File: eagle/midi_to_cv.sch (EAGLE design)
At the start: 36 parts, among them IC1 TL074P, IC4 TL074P, IC5 TL074P, U1 ATMEGA328P_PDIP

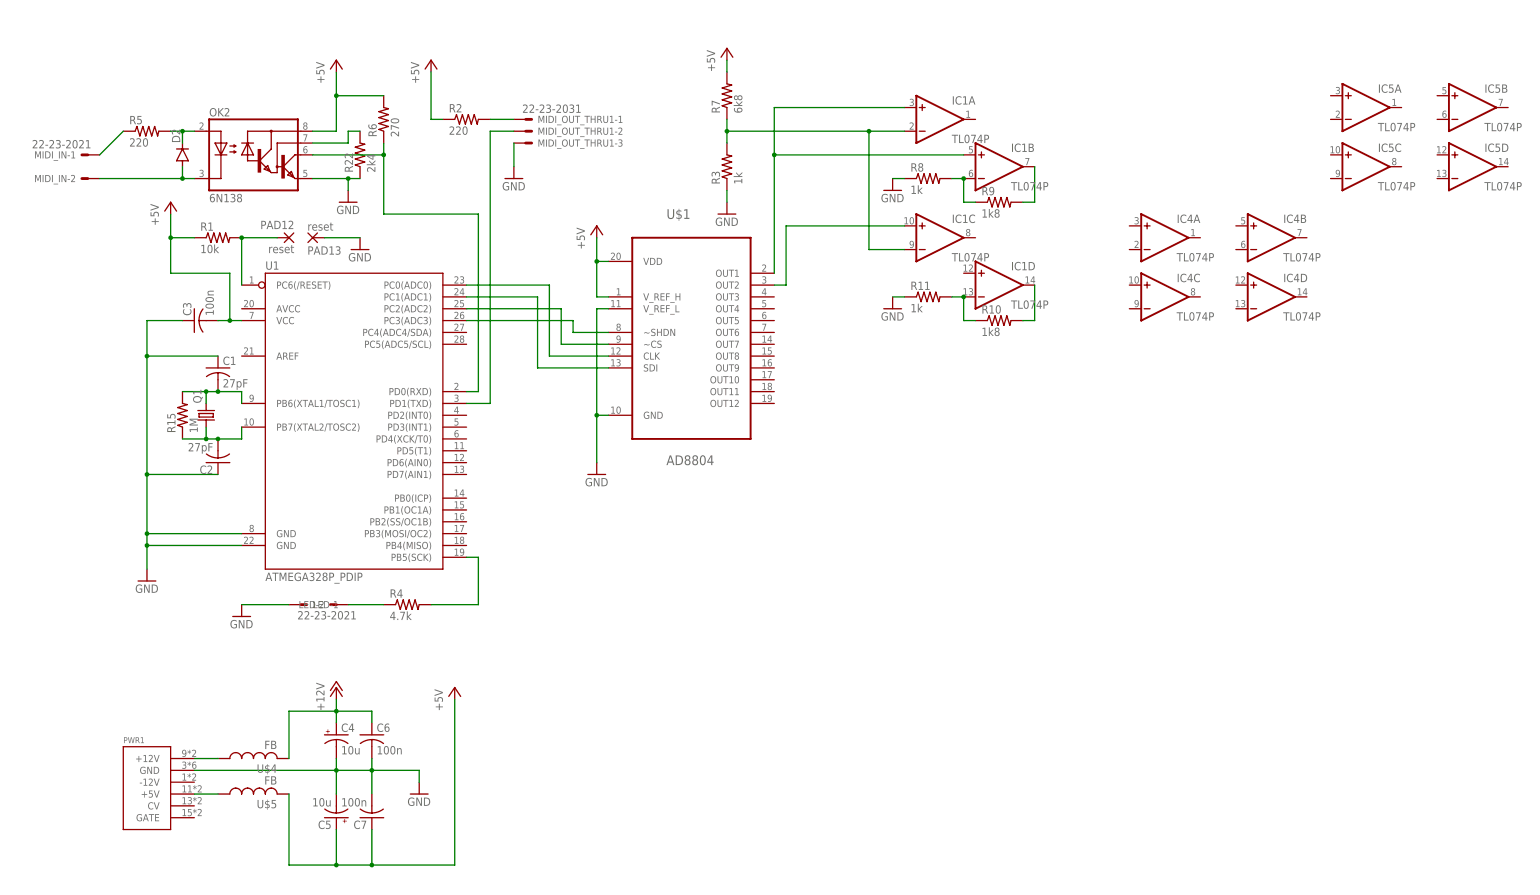
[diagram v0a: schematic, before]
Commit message: routed
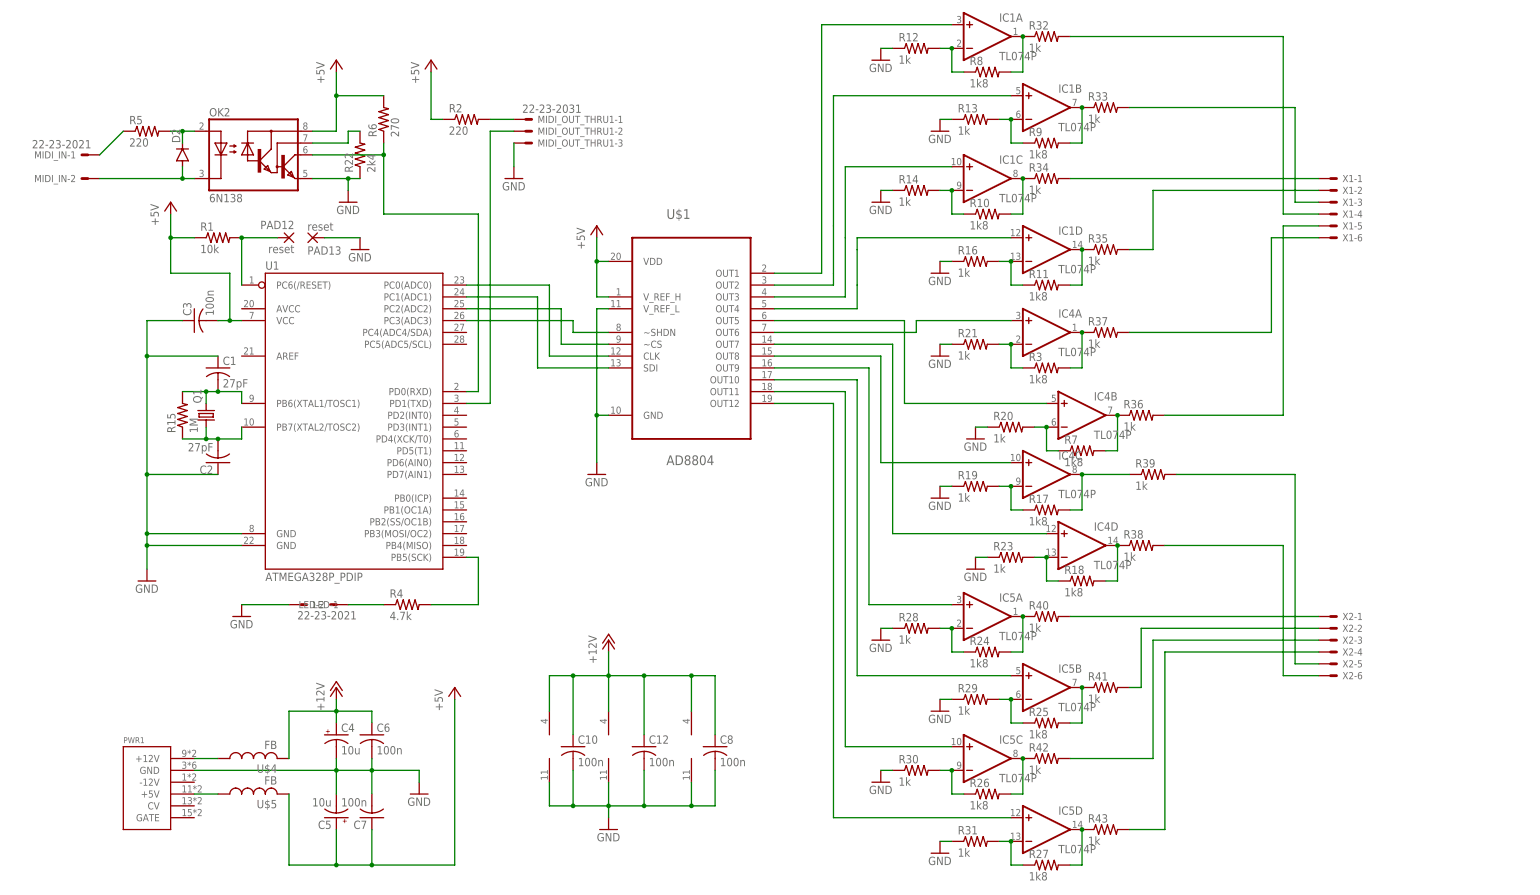
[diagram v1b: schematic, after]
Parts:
- added C10, C12, C8: 100n, rcl:C-US025-024X044
- added R12, R20, R29, R32, R34, R35, R36, R37, R38, R39, R40, R41, R43: 1k, rcl:R-US_0204/7
- added R13, R14, R16, R19, R21, R23, R28, R30, R31, R33, R42: 1k, rcl:R-US_0204/5
- added R17, R18, R24, R25, R26, R27: 1k8, rcl:R-US_0204/2V
- added X1, X2: (no value), con-molex:KK-156-6
- R10, R9: device rcl:R-US_0207/10 -> rcl:R-US_0204/2V
- R11, R3, R8: value 1k -> 1k8; device rcl:R-US_0207/10 -> rcl:R-US_0204/2V
- R5: device rcl:R-US_0207/10 -> rcl:R-US_0204/7
- R7: value 6k8 -> 1k8; device rcl:R-US_0207/10 -> rcl:R-US_0204/2V
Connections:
- new net N$24: IC4C.-IN, R17.1, R19.2
- new net N$25: R34.2, X1-1.S
- new net N$26: IC1A.+IN, U$1.OUT1
- new net N$27: IC1B.+IN, U$1.OUT2
- new net N$28: IC1C.+IN, U$1.OUT3
- new net N$29: IC1D.+IN, U$1.OUT4
- new net N$30: IC4B.-IN, R20.2, R7.1
- new net N$31: IC4A.-IN, R21.2, R3.1
- new net N$32: IC4B.+IN, U$1.OUT5
- new net N$33: IC4A.+IN, U$1.OUT6
- new net N$34: IC4D.+IN, U$1.OUT7
- new net N$35: IC4C.+IN, U$1.OUT8
- new net N$36: IC4D.-IN, R18.1, R23.2
- new net N$37: IC4A.OUT, R3.2, R37.1
- new net N$38: R35.2, X1-2.S
- new net N$39: R33.2, X1-3.S
- new net N$40: R32.2, X1-4.S
- new net N$41: IC5A.+IN, U$1.OUT9
- new net N$42: IC5B.+IN, U$1.OUT10
- new net N$43: IC5C.+IN, U$1.OUT11
- new net N$44: IC5D.+IN, U$1.OUT12
- new net N$45: IC5A.-IN, R24.1, R28.2
- new net N$46: IC5B.-IN, R25.1, R29.2
- new net N$47: IC5C.-IN, R26.1, R30.2
- new net N$48: IC5D.-IN, R27.1, R31.2
- new net N$49: IC5A.OUT, R24.2, R40.1
- new net N$50: IC5B.OUT, R25.2, R41.1
- new net N$51: IC5C.OUT, R26.2, R42.1
- new net N$52: IC5D.OUT, R27.2, R43.1
- new net N$53: IC1A.OUT, R32.1, R8.2
- new net N$54: IC1B.OUT, R33.1, R9.2
- new net N$55: IC1C.OUT, R10.2, R34.1
- new net N$56: IC1D.OUT, R11.2, R35.1
- new net N$57: R36.2, X1-5.S
- new net N$58: R37.2, X1-6.S
- new net N$59: R40.2, X2-1.S
- new net N$61: R41.2, X2-2.S
- new net N$63: R42.2, X2-3.S
- new net N$64: R43.2, X2-4.S
- new net N$65: R39.2, X2-5.S
- new net N$66: R38.2, X2-6.S
- net +12V: now also C10.1, C12.1, C8.1, IC1P.V+, IC4P.V+, IC5P.V+
- net +5V: no longer R7.2
- net GND: now also C10.2, C12.2, C8.2, IC1P.V-, IC4P.V-, IC5P.V-, R12.1, R13.1, R14.1, R16.1, R19.1, R20.1, R21.1, R23.1, R28.1, R29.1, R30.1, R31.1; no longer R11.1, R3.1, R8.1
- net N$13: now also R12.2, R8.1; no longer IC1C.-IN, R3.2, R7.1
- net N$14: now also IC1C.-IN, R10.1, R14.2; no longer IC1A.+IN, IC1B.+IN, U$1.OUT1
- net N$15: now also R13.2; no longer R8.2
- net N$16: now also IC4B.OUT, R36.1, R7.2; no longer IC1B.OUT, R9.2
- net N$21: now also R11.1, R16.2; no longer R10.1, R11.2
- net N$22: now also IC4C.OUT, R17.2, R39.1; no longer IC1C.+IN, U$1.OUT2
- net N$23: now also IC4D.OUT, R18.2, R38.1; no longer IC1D.OUT, R10.2
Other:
- moved on the sheet: IC1A, IC1B, IC1C, IC1D, IC4A, IC4B, IC4C, IC4D, IC5A, IC5B, IC5C, IC5D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

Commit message: tweaks
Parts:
- R29, R35, R41: device rcl:R-US_0204/7 -> rcl:R-US_0204/5
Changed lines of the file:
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@@
 <part name="R27" library="rcl" deviceset="R-US_" device="0204/2V" value="1k8"/>
 <part name="R28" library="rcl" deviceset="R-US_" device="0204/5" value="1k"/>
-<part name="R29" library="rcl" deviceset="R-US_" device="0204/7" value="1k"/>
+<part name="R29" library="rcl" deviceset="R-US_" device="0204/5" value="1k"/>
 <part name="R30" library="rcl" deviceset="R-US_" device="0204/5" value="1k"/>
 <part name="R31" library="rcl" deviceset="R-US_" device="0204/5" value="1k"/>
@@
 <part name="R33" library="rcl" deviceset="R-US_" device="0204/5" value="1k"/>
 <part name="R34" library="rcl" deviceset="R-US_" device="0204/7" value="1k"/>
-<part name="R35" library="rcl" deviceset="R-US_" device="0204/7" value="1k"/>
+<part name="R35" library="rcl" deviceset="R-US_" device="0204/5" value="1k"/>
 <part name="R36" library="rcl" deviceset="R-US_" device="0204/7" value="1k"/>
 <part name="R37" library="rcl" deviceset="R-US_" device="0204/7" value="1k"/>
@@
 <part name="R39" library="rcl" deviceset="R-US_" device="0204/7" value="1k"/>
 <part name="R40" library="rcl" deviceset="R-US_" device="0204/7" value="1k"/>
-<part name="R41" library="rcl" deviceset="R-US_" device="0204/7" value="1k"/>
+<part name="R41" library="rcl" deviceset="R-US_" device="0204/5" value="1k"/>
 <part name="R42" library="rcl" deviceset="R-US_" device="0204/5" value="1k"/>
 <part name="R43" library="rcl" deviceset="R-US_" device="0204/7" value="1k"/>
